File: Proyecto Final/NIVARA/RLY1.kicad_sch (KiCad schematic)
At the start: 0 parts

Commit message: Actualización
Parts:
- added K1, K2: DS1E-S-DC3V, Relay DS1E:RELAY_DS1E_PAN, symbol DS1E-S-DC3V:DS1E-S-DC3V
- added U3: LK1802, Easy Eda:LK1802, symbol Easy Eda:LK1802
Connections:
- new net: K2.6 (COIL-), U3.6 (2C)
- new net: K1.6 (COIL-), U3.1 (1C)
- new net +3.3V: K1.1 (COIL+), K2.1 (COIL+)
- new net GND: U3.2 (E)
- new net OnRLY-1: U3.3 (1B)
- new net OnRLY-2: U3.4 (2B)
- new net RLY1_COMÚN: K1.7 (COM)
- new net RLY1_NC: K1.10 (NC)
- new net RLY1_NO: K1.12 (NO)
- new net RLY2_COMÚN: K2.7 (COM)
- new net RLY2_NC: K2.10 (NC)
- new net RLY2_NO: K2.12 (NO)
- new net VCC: U3.5 (COM)

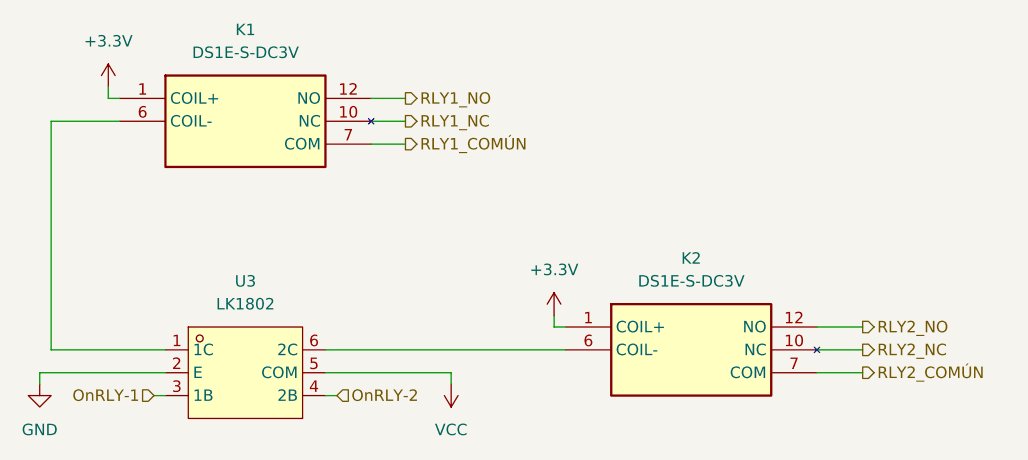
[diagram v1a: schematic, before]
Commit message: Actualización
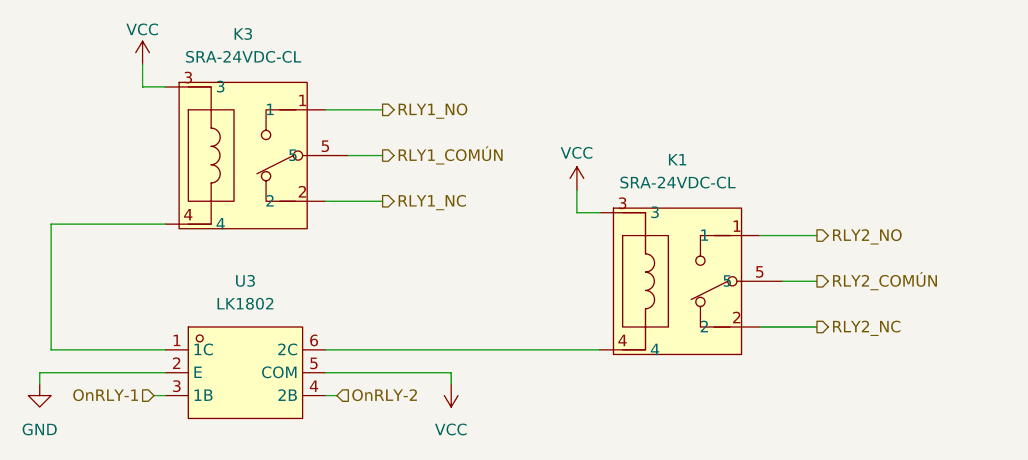
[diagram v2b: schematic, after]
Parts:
- removed K1, K2: DS1E-S-DC3V, Relay DS1E:RELAY_DS1E_PAN, symbol DS1E-S-DC3V:DS1E-S-DC3V
- added K1, K3: SRA-24VDC-CL, EasyEDA:RELAY-TH_SRA-X-CX, symbol Easy:SRA-24VDC-CL
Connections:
- net RLY1_COMÚN: now also K3.5
- net RLY1_NC: now also K3.2
- net RLY1_NO: now also K3.1
- net RLY2_COMÚN: now also K1.5
- net RLY2_NC: now also K1.2
- net RLY2_NO: now also K1.1
- net VCC: now also K1.3, K3.3
- net at U3.6 (2C): now also K1.4
- net at U3.1 (1C): now also K3.4

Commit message: Avances en PCB
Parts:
- K1, K3: footprint EasyEDA:RELAY-TH_SRA-X-CX -> Easy Eda:RELAY-TH_SRA-X-CX
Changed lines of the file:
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@@
 			)
 		)
-		(property "Footprint" "EasyEDA:RELAY-TH_SRA-X-CX"
+		(property "Footprint" "Easy Eda:RELAY-TH_SRA-X-CX"
 			(at 82.55 49.53 0)
 			(effects
@@
 			)
 		)
-		(property "Footprint" "EasyEDA:RELAY-TH_SRA-X-CX"
+		(property "Footprint" "Easy Eda:RELAY-TH_SRA-X-CX"
 			(at 130.81 63.5 0)
 			(effects
